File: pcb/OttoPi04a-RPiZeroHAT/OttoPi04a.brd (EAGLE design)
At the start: 65 x 55 mm, 26 parts

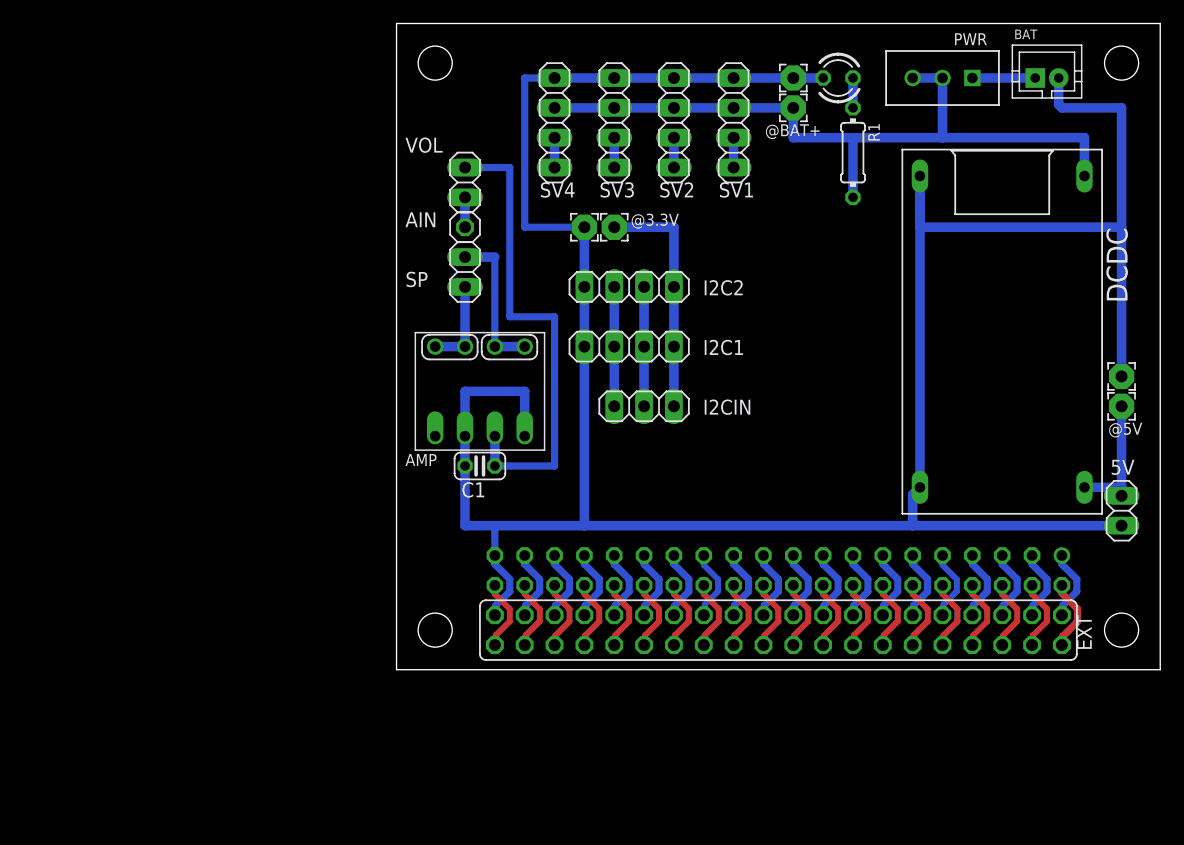
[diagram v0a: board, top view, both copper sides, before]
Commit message: update
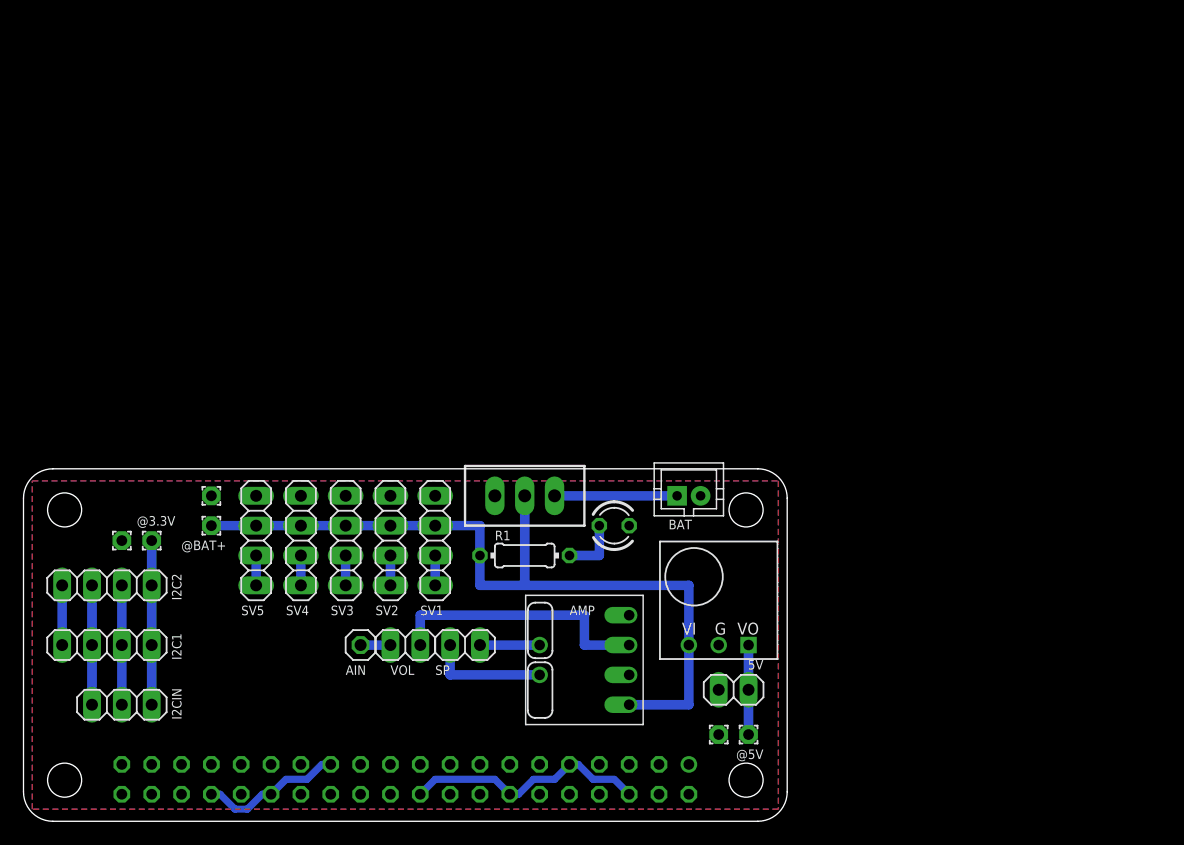
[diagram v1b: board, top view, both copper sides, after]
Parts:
- removed C1: (no value), rcl:C025-024X044
- removed DCDC: (no value), ytani1:DCDC-5V_28V-2A
- removed EXT: (no value), con-lstb:MA20-2W
- removed G5V: (no value), wirepad:2,15/1,0
- removed PWR: (no value), ytani1:SW3-1
- added DCDC1: (no value), ytani1:DCDC-5V-0.48A
- added PAD2: (no value), wirepad:1,6/0,9
- added SV5: (no value), pinhead:1X04
- added SW: TL36PO, switch:TL3XPO
- @3.3V, @5V, @BAT+, PAD4, PAD6: device wirepad:2,15/1,0 -> wirepad:1,6/0,9
- AMP: device ytani1:PAM8012MOD -> ytani1:PAM8012MOD-A
- moved @BAT+ 61.0 mm to (-16.5, 10.2)
- moved PAD6 61.0 mm to (-16.5, 12.7)
- moved I2C1 51.2 mm to (-25.4, 0.00)
- moved I2C2 51.2 mm to (-25.4, 5.08)
- moved I2CIN 51.2 mm to (-24.1, -5.08)
- moved @3.3V 47.6 mm to (-21.6, 8.89)
- moved PAD4 47.6 mm to (-24.1, 8.89)
- moved BAT 46.8 mm to (24.1, 12.7)
- moved R1 44.2 mm to (10.2, 7.62), turned to 180 degrees
- moved SV1 43.7 mm to (2.54, 8.89)
- moved SV2 43.0 mm to (-1.27, 8.89)
- moved LED1 42.6 mm to (17.8, 10.2), turned to 0 degrees
- moved @5V 42.3 mm to (29.2, -7.62)
- moved SV3 42.3 mm to (-5.08, 8.89)
- moved SV4 41.6 mm to (-8.89, 8.89)
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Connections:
- removed net AIN1: AIN.1, VOL.1
- removed net BAT+: @BAT+.1, DCDC.VIN+, PWR.2, PWR.3, R1.2, SV1.2, SV2.2, SV3.2, SV4.2
- removed net BAT+S: BAT.1, PWR.1
- removed net GND14: EXT.14, RPI.14
- removed net GND20: EXT.20, RPI.20
- removed net GND25: EXT.25, RPI.25
- removed net GND30: EXT.30, RPI.30
- removed net GND34: EXT.34, RPI.34
- removed net GND6: EXT.6, RPI.6
- removed net GND9: EXT.9, RPI.9
- new net +4V_S: BAT.1, SW.1
- new net N$1: AIN.1, VOL.2
- new net SV5: SV5.3, SV5.4
- net +3V3-S1: no longer EXT.1
- net +3V3-S2: no longer EXT.17
- net +5V: now also 5V.2, DCDC1.+5V; no longer 5V.1, DCDC.VOUT+
- net +5V-S1: no longer EXT.2
- net +5V-S2: no longer EXT.4
- net AIN: now also VOL.1; no longer C1.1, VOL.2
- net GND: now also 5V.1, DCDC1.GND, PAD2.1, RPI.14, RPI.20, RPI.25, RPI.30, RPI.34, RPI.6, RPI.9, SV5.1; no longer 5V.2, C1.2, DCDC.VIN-, DCDC.VOUT-, EXT.39, G5V.1
- net GPIO0: no longer EXT.27
- net GPIO1: no longer EXT.28
- net GPIO10: no longer EXT.19
- net GPIO11: no longer EXT.23
- net GPIO12: no longer EXT.32
- net GPIO13: no longer EXT.33
- net GPIO14: no longer EXT.8
- net GPIO15: no longer EXT.10
- net GPIO16: no longer EXT.36
- net GPIO17: no longer EXT.11
- net GPIO18: no longer EXT.12
- net GPIO19: no longer EXT.35
- net GPIO20: no longer EXT.38
- net GPIO21: no longer EXT.40
- net GPIO22: no longer EXT.15
- net GPIO23: no longer EXT.16
- net GPIO24: no longer EXT.18
- net GPIO25: no longer EXT.22
- net GPIO26: no longer EXT.37
- net GPIO27: no longer EXT.13
- net GPIO4: no longer EXT.7
- net GPIO5: no longer EXT.29
- net GPIO6: no longer EXT.31
- net GPIO7: no longer EXT.26
- net GPIO8: no longer EXT.24
- net GPIO9: no longer EXT.21
- net SCL-S: no longer EXT.5
- net SDA-S: no longer EXT.3
- net SP+: no longer AMP.SP+@2
- net SP-: no longer AMP.SP-@2
- net V+: now also @BAT+.1, DCDC1.VIN, R1.2, SV1.2, SV2.2, SV3.2, SV4.2, SV5.2, SW.2
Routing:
- net GND: track 235.6 -> 38.6 mm
- net V+: track 0.00 -> 68.6 mm
- net BAT+: track 63.6 -> 0.00 mm
- net AIN: track 40.6 -> 22.9 mm
- net +4V_S: track 0.00 -> 10.4 mm
- net SP-: track 12.7 -> 5.08 mm
- net +3V3: track 20.3 -> 14.0 mm
- net +5V-S1: track 6.15 -> 0.00 mm
- net GPIO18: track 6.11 -> 0.00 mm
- net GPIO17: track 6.11 -> 0.00 mm
- net GPIO7: track 6.11 -> 0.00 mm
- net SCL-S: track 6.11 -> 0.00 mm
- net GPIO4: track 6.11 -> 0.00 mm
- net GPIO13: track 6.11 -> 0.00 mm
- net GPIO8: track 6.11 -> 0.00 mm
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- added copper zone on layer 1, net GND
- added copper zone on layer 16, net GND
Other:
- board size 65 x 55 mm -> 65 x 30 mm
